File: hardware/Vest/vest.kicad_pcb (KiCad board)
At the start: 2 copper layers, 152.4 x 101.6 mm, 47 parts, among them P1 USB_B, P2 USB_B_Power, Q1 MMBT3904, Q2 MMBT3904

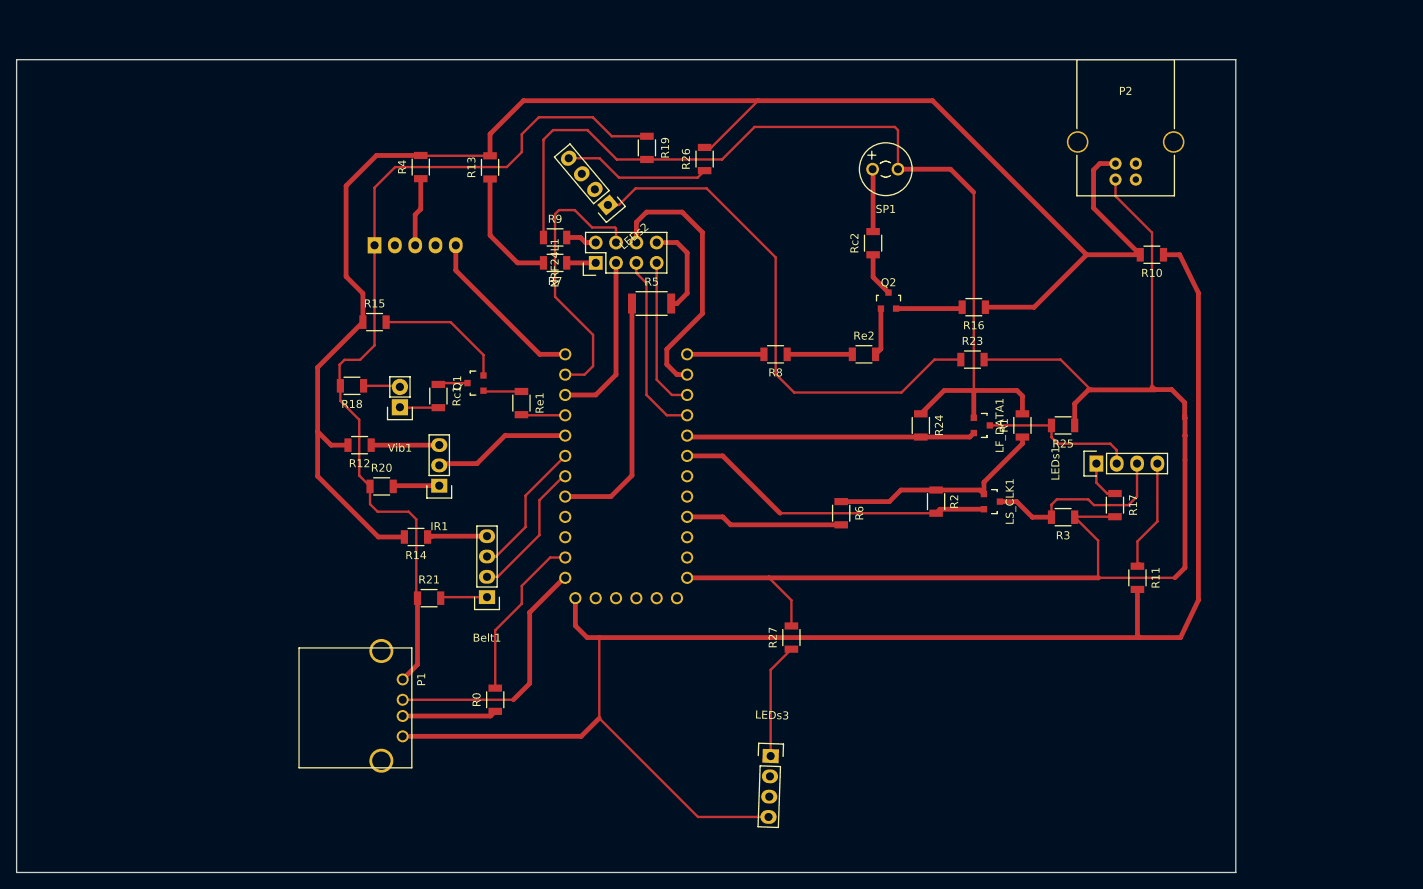
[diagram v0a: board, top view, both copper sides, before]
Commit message: updated pcb
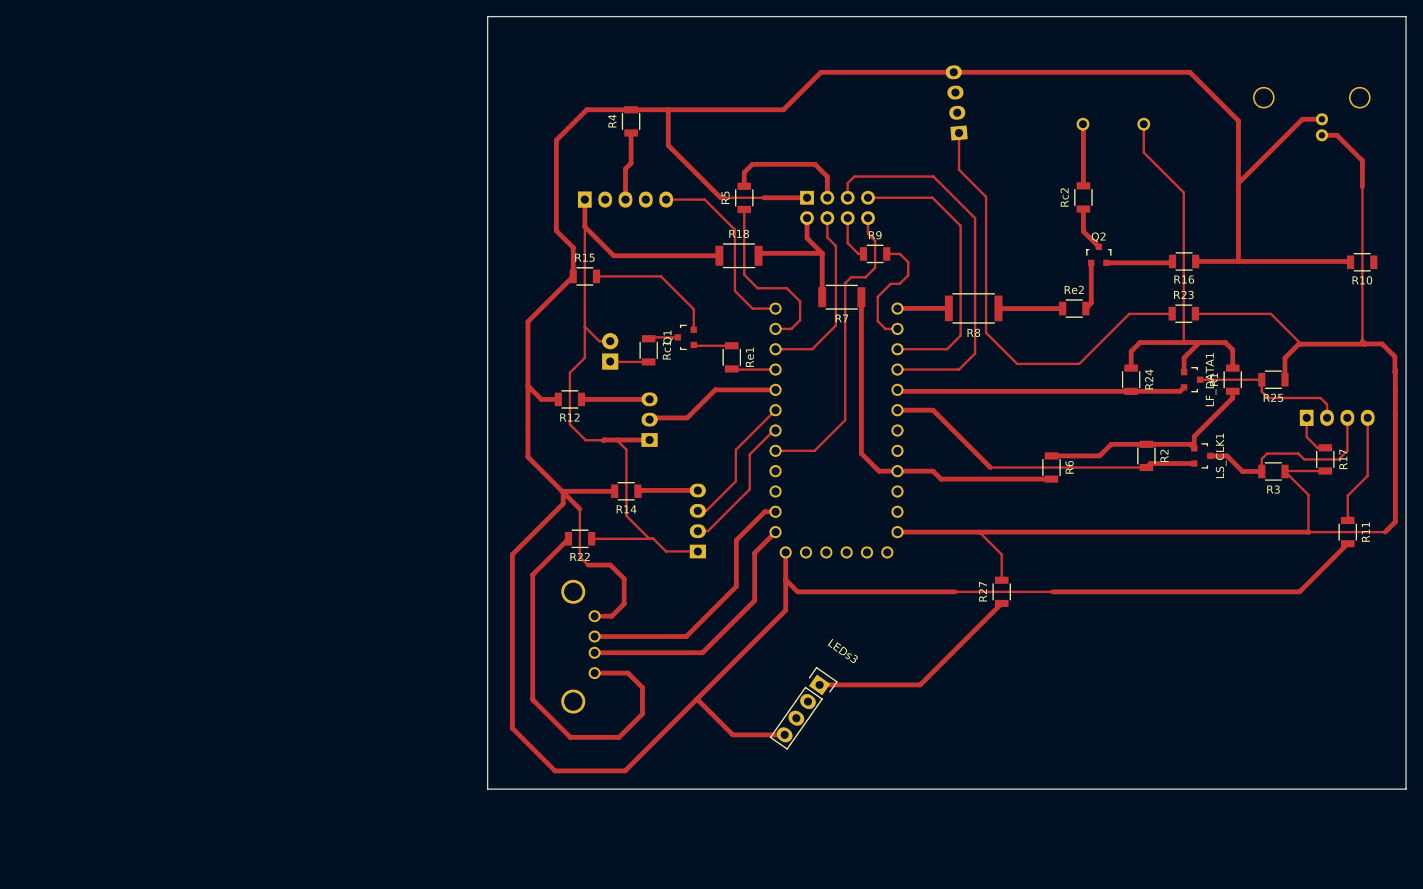
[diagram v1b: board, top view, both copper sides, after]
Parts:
- removed R0: R0, Resistors_SMD:R_1206
- removed R13, R26: 0, Resistors_SMD:R_1206
- removed R19, R20, R21: R, Resistors_SMD:R_1206
- added R22: 0, Resistors_SMD:R_1206, F.Cu at (95.8, 113.2)
- Belt1, IR1, LEDs1, LEDs2, NRF24L1, P1, P2, Vib1: moved to B.Cu
- R18, R7: footprint Resistors_SMD:R_1206 -> Resistors_SMD:R_2010
- R5: footprint Resistors_SMD:R_2010 -> Resistors_SMD:R_1206
- R8: footprint Resistors_SMD:R_1206 -> Resistors_SMD:R_2512
- SP1: footprint Buzzers_Beepers:MagneticBuzzer_Kingstate_KCG0601 -> Buzzers_Beepers:MagneticBuzzer_ProSignal_ABI-010-RC; moved to B.Cu
- moved R18 51.0 mm to (115.7, 77.9), turned to 0 degrees
- moved LEDs2 44.8 mm to (143.2, 62.5), turned to 5 degrees
- moved R9 40.1 mm to (132.7, 77.6)
- moved R7 36.1 mm to (128.5, 83.0)
- moved SP1 31.2 mm to (166.3, 61.4)
- moved NRF24L1 27.6 mm to (124.2, 70.6), turned to 270 degrees
- moved R23 27.0 mm to (171.3, 85.1)
- moved Belt1 27.0 mm to (110.6, 114.8), turned to 0 degrees
- moved LEDs1 26.9 mm to (186.7, 98.1), turned to 270 degrees
- moved LS_CLK1 26.9 mm to (173.6, 102.9)
- moved R1 26.9 mm to (177.4, 93.3)
- moved R16 26.9 mm to (171.3, 78.6)
- moved R17 26.9 mm to (189.0, 103.3)
- moved R6 26.9 mm to (154.8, 104.3)
- moved IR1 26.9 mm to (104.5, 100.9), turned to 0 degrees
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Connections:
- Belt1 pad 1: Belt_VCC_OUT -> VCC
- IR1 pad 1: Buzzer_VCC_OUT -> VCC
- LEDs2 pad 4: Net-(LEDs2-Pad4) -> GND
- Mic1 pad 1: VCC_J -> VCC
- NRF24L1 pad 1: Net-(NRF24L1-Pad1) -> GND
- NRF24L1 pad 2: Net-(NRF24L1-Pad2) -> VCC
- NRF24L1 pad 8: Net-(NRF24L1-Pad8) -> IRQ
- P1 pad 1: VCC_J -> Net-(P1-Pad1)
- P1 pad 3: Net-(P1-Pad3) -> RX_to_weapon_TX
- R18 pad 1: Vib_VCC_OUT -> VCC
- R18 pad 2: VCC_J -> VCC
- R5 pad 1: IRQ -> Net-(R5-Pad1)
- R5 pad 2: Net-(NRF24L1-Pad8) -> CE
- R7 pad 1: Net-(NRF24L1-Pad1) -> VCC
- R7 pad 2: Net-(R13-Pad1) -> VCC
- R9 pad 1: VCC -> MOSI
- R9 pad 2: Net-(NRF24L1-Pad2) -> Net-(R9-Pad2)
- Vib1 pad 2: Vib_VCC_OUT -> VCC
- uP1 pad 16: CE -> CSN
- uP1 pad 17: CSN -> Net-(R5-Pad1)
- uP1 pad 29: MOSI -> Net-(R9-Pad2)
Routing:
- net VCC_J: track 111.2 -> 0.00 mm
- net VCC: track 168.5 -> 233.7 mm
- net Net-(P1-Pad1): track 0.00 -> 48.9 mm
- net MOSI: track 33.8 -> 5.67 mm
- net SCK: track 23.2 -> 47.7 mm
- net Net-(R5-Pad1): track 0.00 -> 22.4 mm
- net Net-(LEDs2-Pad4): track 18.4 -> 0.00 mm
- net MISO: track 19.2 -> 35.4 mm
- net Net-(R9-Pad2): track 0.00 -> 15.6 mm
- net Net-(R13-Pad1): track 15.2 -> 0.00 mm
- net CSN: track 35.4 -> 22.6 mm
- net Net-(LEDs3-Pad1): track 14.4 -> 27.0 mm
- net Net-(LEDs2-Pad1): track 65.8 -> 53.7 mm
- net Net-(NRF24L1-Pad8): track 11.9 -> 0.00 mm
- net Net-(P1-Pad3): track 11.8 -> 0.00 mm
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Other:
- board size 152.4 x 101.6 mm -> 114.8 x 96.6 mm
